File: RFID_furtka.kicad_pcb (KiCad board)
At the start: 2 copper layers, 20 parts, among them J1 CONN_01X03, Q1 SI2300DS, SW1 TSC_RELAY, U1 LDF33DT-TR, U2 MFRC522, U3 nodemcu-devkit-v1.0(ESP8266)

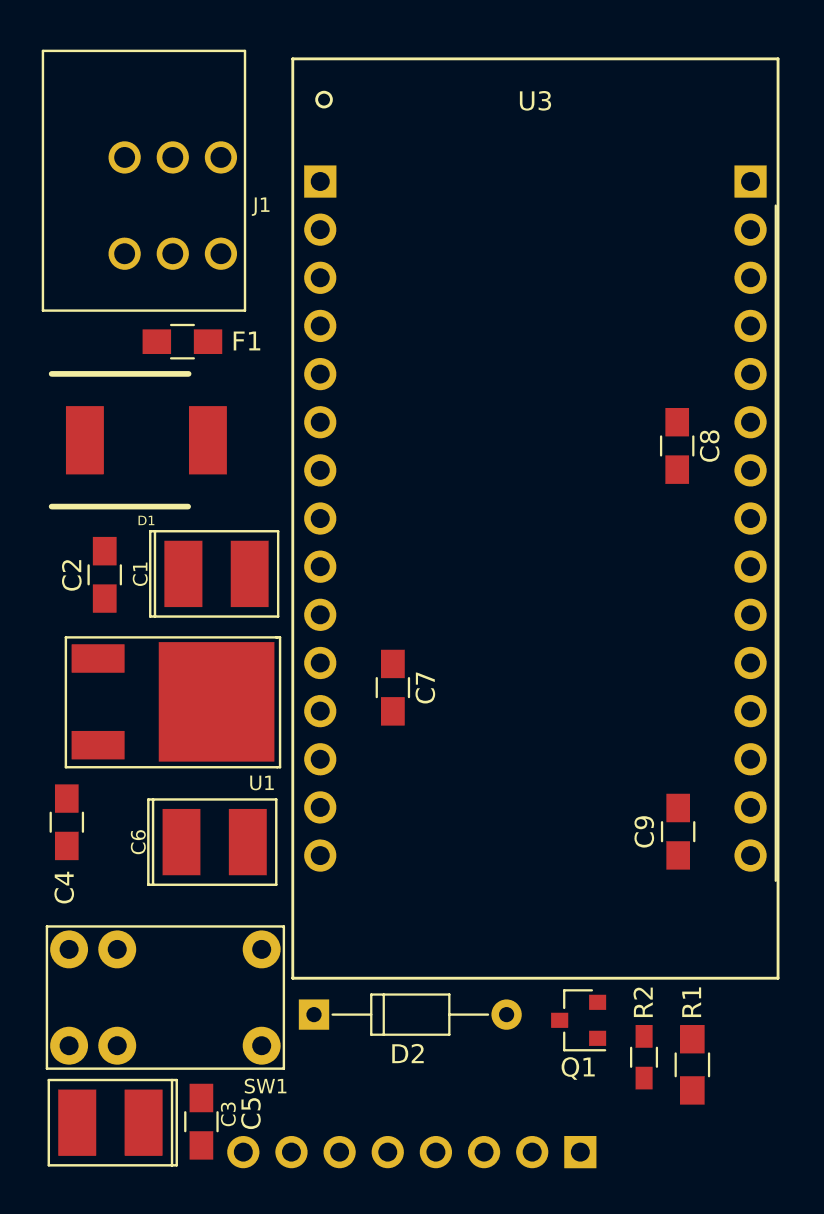
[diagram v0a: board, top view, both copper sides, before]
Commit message: Add BOM
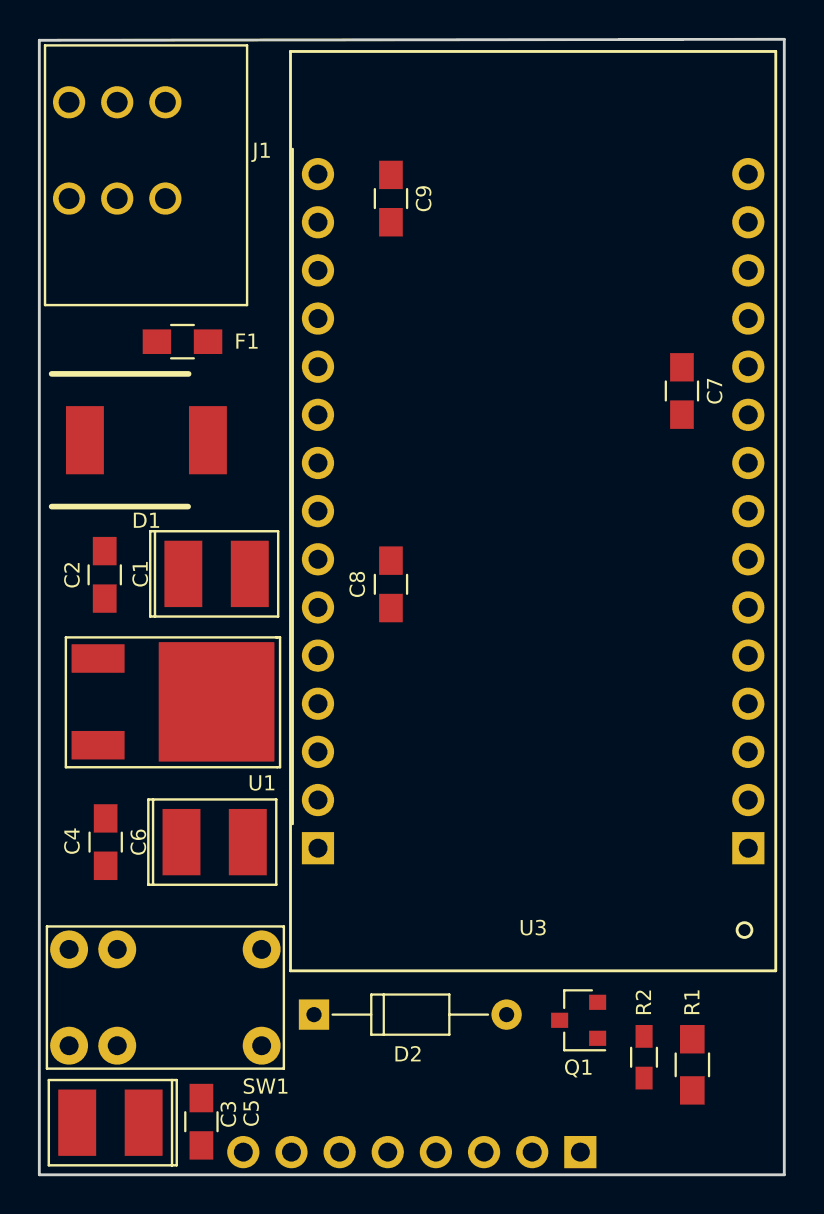
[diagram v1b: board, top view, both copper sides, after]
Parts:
- moved C9 36.7 mm to (147.4, 83.5), turned to 270 degrees
- moved C7 21.9 mm to (162.8, 93.6)
- moved C8 16.8 mm to (147.4, 103.8), turned to 90 degrees
- moved J1 4.13 mm to (133.0, 80.9), turned to 0 degrees
- moved C4 2.30 mm to (132.3, 117.4)
- moved U3 0.41 mm to (154.9, 99.9), turned to 180 degrees
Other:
- board outline added: 39.3 x 59.9 mm
- net class Default: clearance 0.2 -> 0.2032; trace_width 0.25 -> 0.254
- rule trace_clearance: 0.2 -> 0.2032
- rule trace_min: 0.2 -> 0.2032
- rule via_min_drill: 0.3 -> 0.4
- rule via_min_size: 0.4 -> 0.6
